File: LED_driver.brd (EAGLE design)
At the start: 32.2 x 30 mm, 17 parts

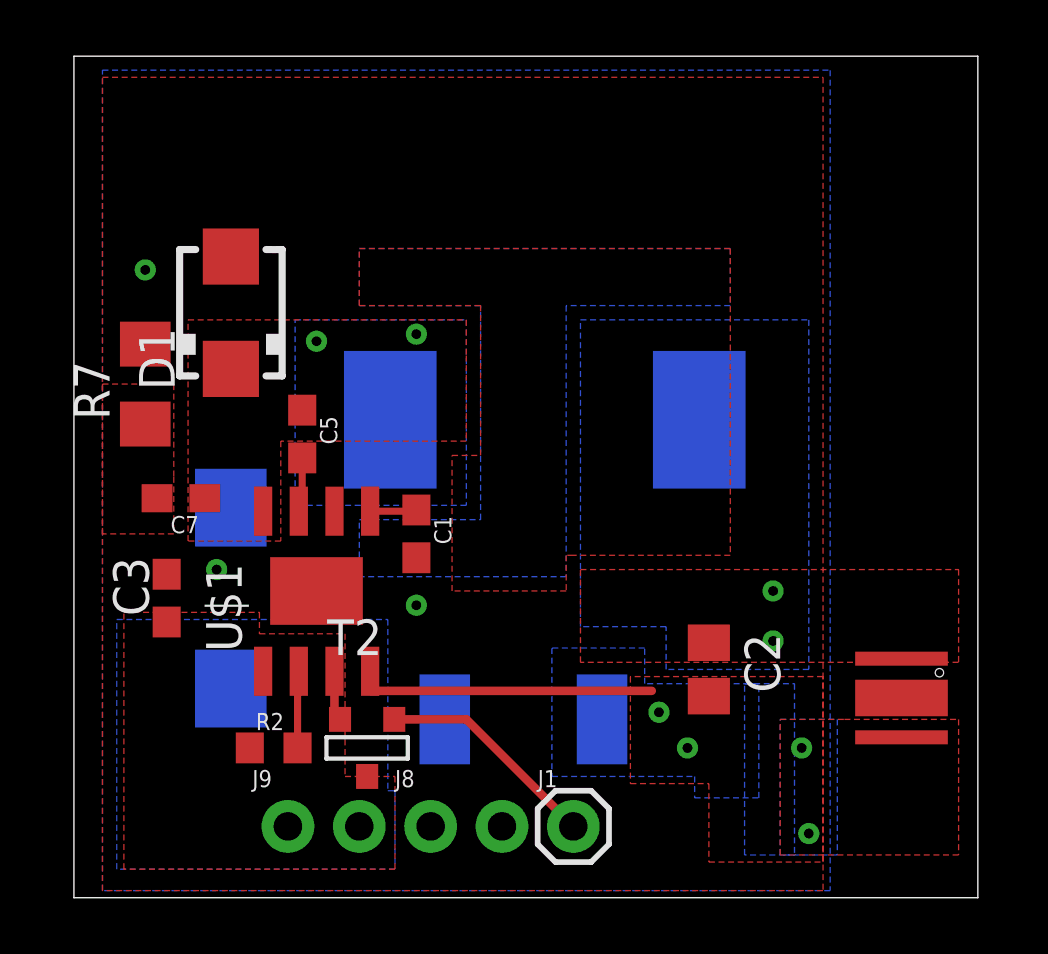
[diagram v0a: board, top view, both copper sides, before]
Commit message: continued revisions
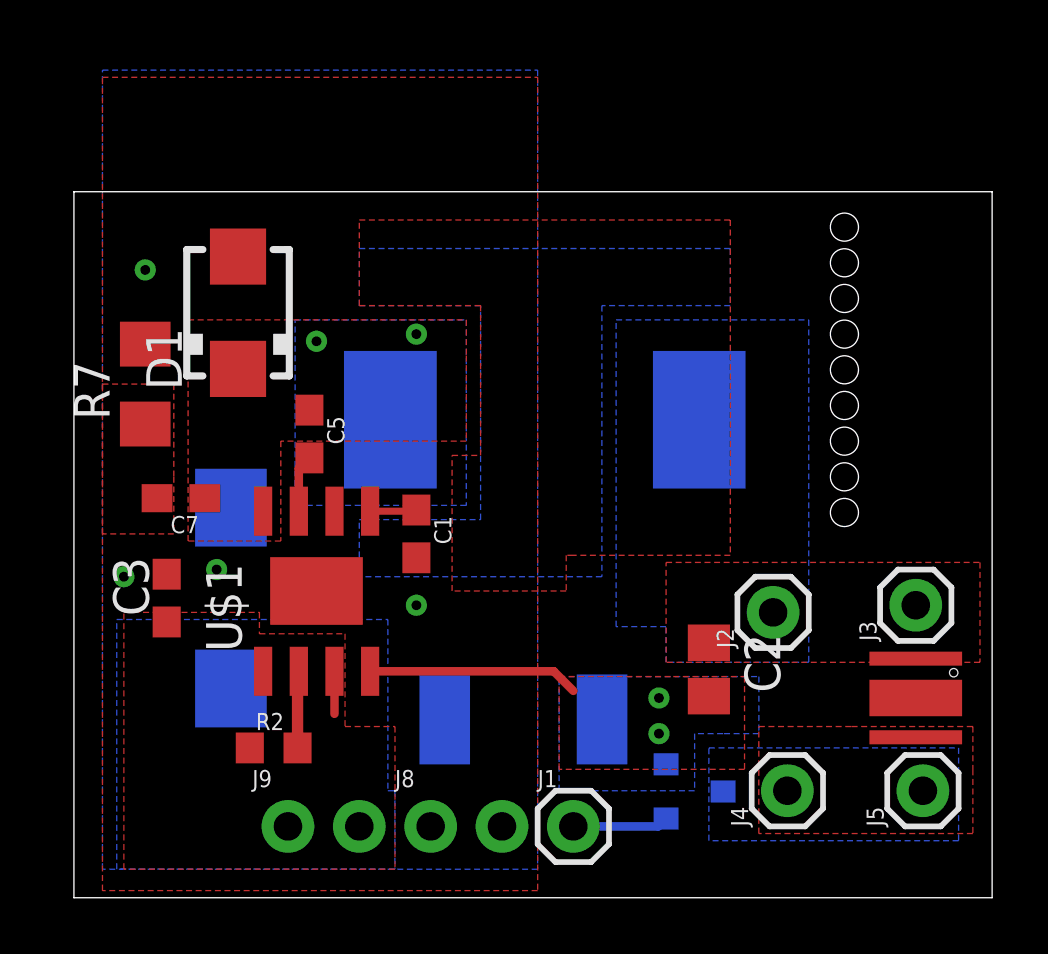
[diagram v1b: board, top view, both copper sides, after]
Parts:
- added J2, J3, J4, J5: (no value), SparkFun-Connectors:1X01
- moved T2 11.8 mm to (22.1, 3.81), flipped to the bottom, turned to 270 degrees
- moved U$3 0.51 mm to (30.0, 7.11)
- moved C5 0.25 mm to (8.38, 16.5)
- moved D1 0.25 mm to (5.84, 20.8)
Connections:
- removed net N$7: T2.2, U$1.3
- new net N$3: J4.1, J5.1, T2.1, U$3.LED-
- net 12V: now also U$1.3; no longer T2.1
- net LED+: now also J2.1, J3.1
- net LED-: now also T2.2; no longer U$3.LED-
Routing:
- net LED_PWM: track 8.49 -> 3.42 mm
- net LED-: track 10.7 -> 8.22 mm, vias 4 -> 2
- net N$7: track 1.79 -> 0.00 mm
- net 12V: track 0.00 -> 1.51 mm
- added copper zone on layer 1, net N$3
- added copper zone on layer 16, net N$3
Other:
- board size 32.2 x 30 mm -> 32.7 x 25.1 mm
